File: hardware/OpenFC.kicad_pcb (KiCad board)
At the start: 6 copper layers, 38.9 x 38.9 mm, 168 parts, among them CN1 SM04B-SRSS-TB, J1 5V, J10 5V, J11 5V, J12 5V, J13 5V, J14 5V, J15 5V, J16 5V, J17 5V, J18 5V, J19 5V, J2 5V, J20 5V, J21 5V, J22 5V, J23 5V, J24 5V, J25 5V, J26 5V, J27 5V, J28 5V, J29 5V, J3 5V, J30 5V, J31 5V, J32 5V, J33 5V, J34 5V, J35 5V, J36 5V, J37 5V, J38 5V, J39 5V, J4 5V, J40 5V, J41 5V, J42 5V, J43 5V, J44 5V, J47 5V, J48 5V, J49 5V, J5 5V, J50 5V, J51 5V, J52 5V, J53 5V, J54 5V, J55 5V, J6 5V, J7 5V, J8 5V, J9 5V, P1 SM08B-SRSS-TB(LF)(SN), Q1 AP1606, Q2 AP1606, U1 TS2306A 240GF MSM 9_C2976675, U10 SN74LVC1G3157DTBR, U11 COS8051SOT, U12 TLV7031DPWR, U13 SM03B-SRSS-TB, U14 SM06B-SRSS-TB(LF)(SN), U2 RP2354B_C39843328, U3 TI LMR51430YFDDCR, U4 TI LMR51430YFDDCR, U5 TPS2116DRLR, U6 NCV8187AMT180TAG, U7 LP5912-3.3DRVR, U8 SM06B-SRSS-TB(LF)(SN), U9 LSM6DSV16XTR, X1 XTM25012000JT00351001

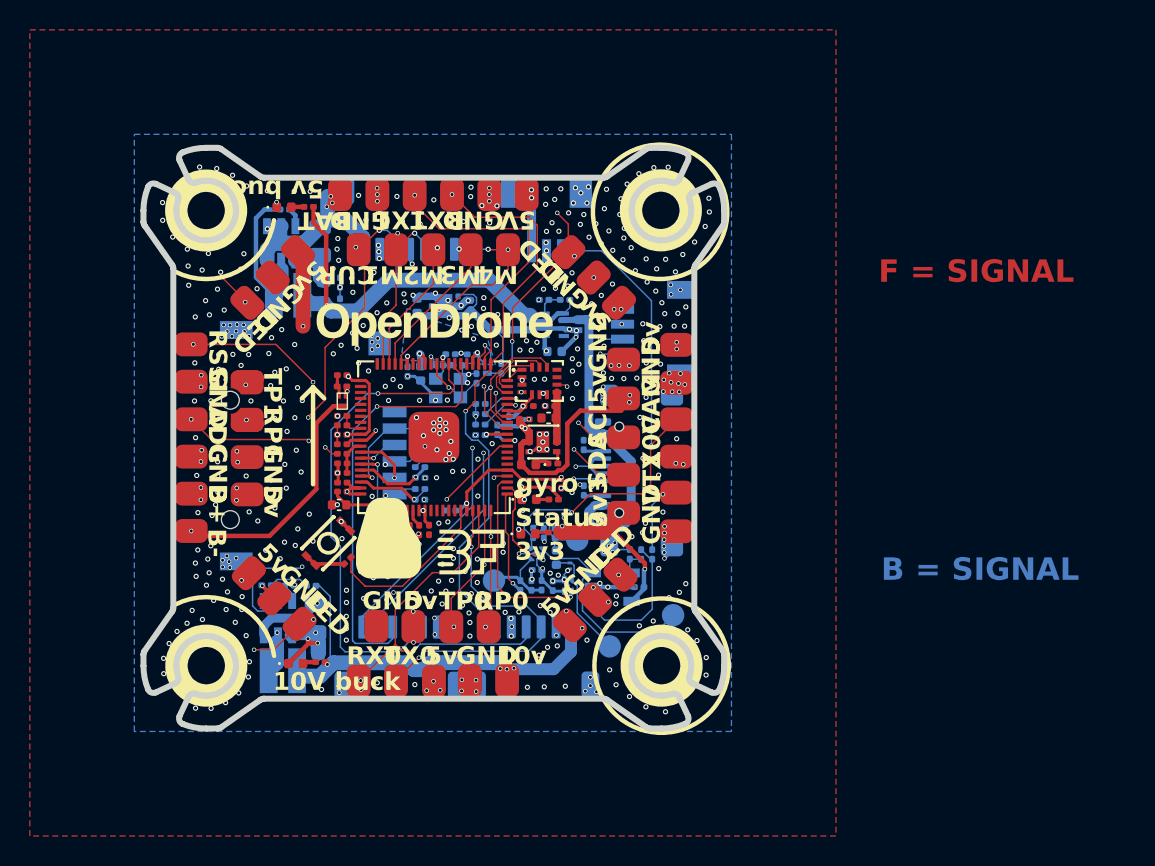
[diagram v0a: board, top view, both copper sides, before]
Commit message: my changes purchared pcb
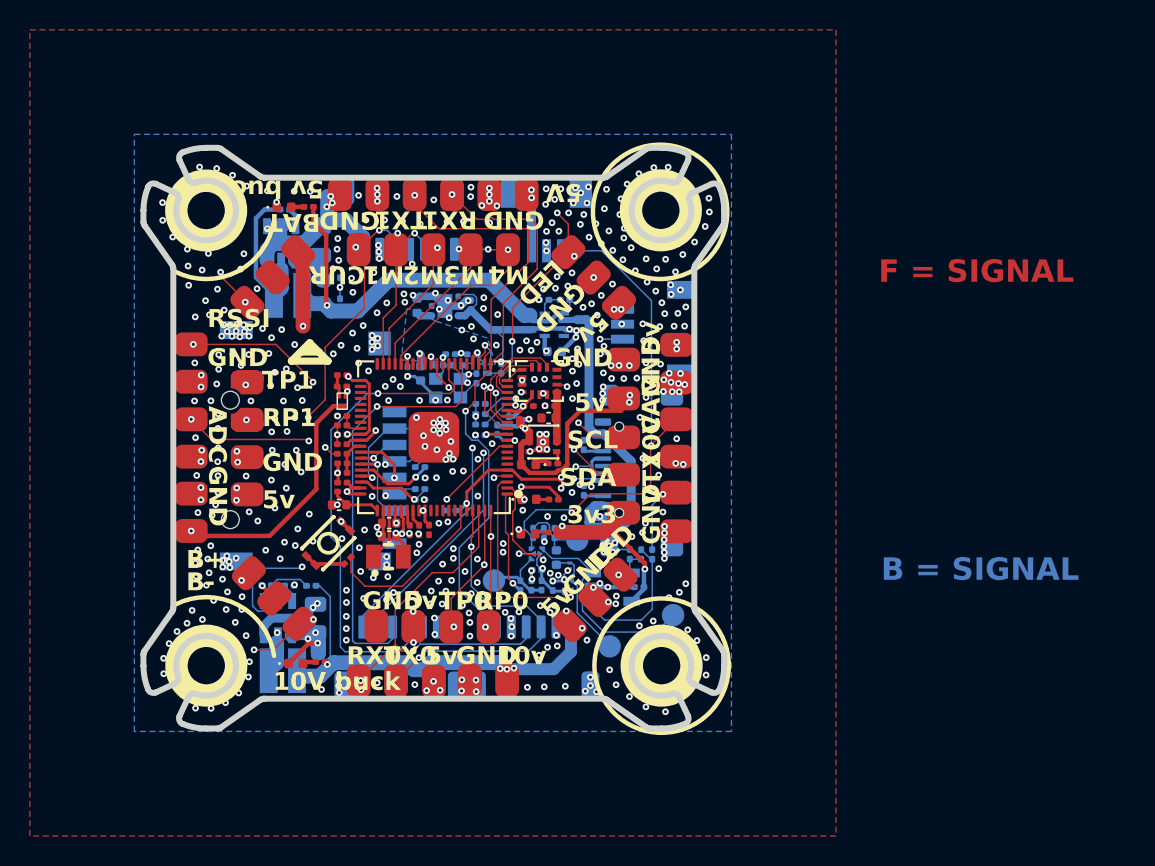
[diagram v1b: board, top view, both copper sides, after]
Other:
- board text removed: "FC"
- board text removed: "Open"
- board text removed: "SBUS"
- board text removed: "Status"
- board text removed: "TEL"
- board text removed: "gyro"
- board text removed: "lite"
